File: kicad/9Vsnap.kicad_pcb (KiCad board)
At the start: 2 copper layers, 26 x 17 mm, 11 parts, among them P1 9V_IN, P2 OUT, U1 LM317EMP

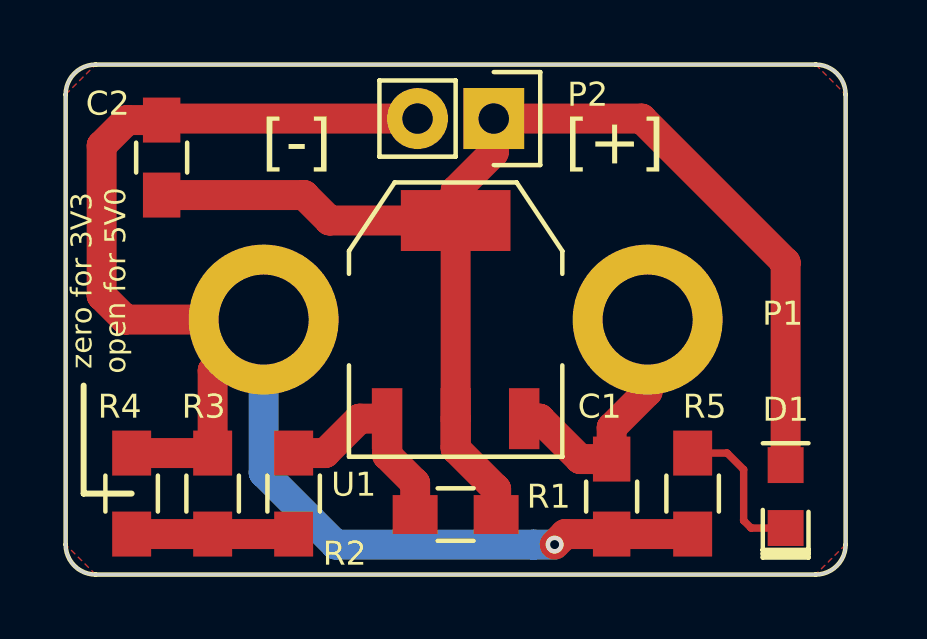
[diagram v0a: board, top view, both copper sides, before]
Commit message: Done. Gerbers ready
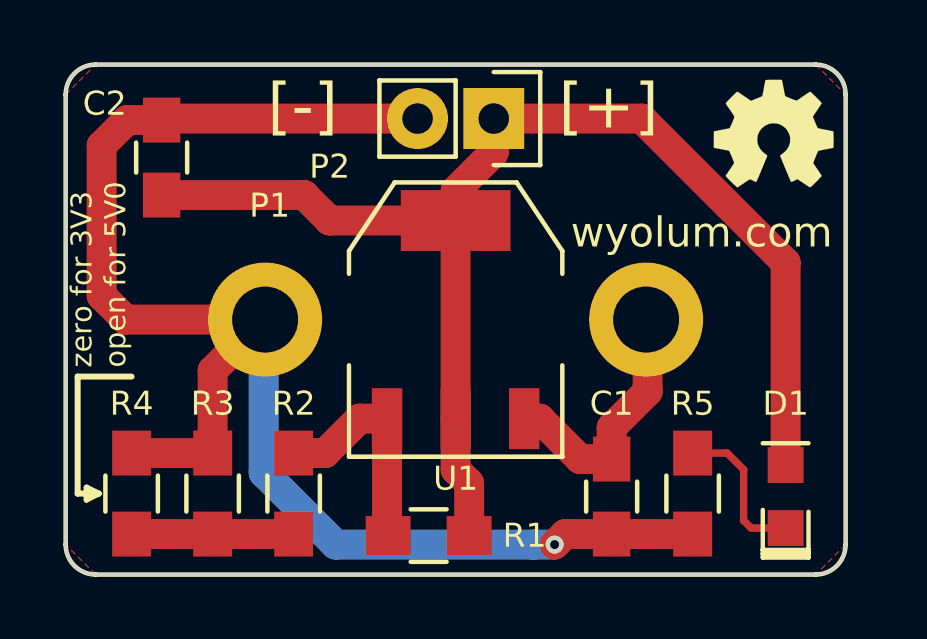
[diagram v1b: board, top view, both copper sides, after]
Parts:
- added G***: LOGO, 9Vsnap:OSHW_logo_notext, B.Cu at (100.0, 102.5)
- added G***: LOGO, 9Vsnap:OSHW_logo_notext, F.Cu at (110.6, 93.8)
- P1: footprint 9Vsnap:9V_clip -> 9Vsnap:9V_clip_968
- moved R1 1.14 mm to (99.1, 107.2)
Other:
- board text added: "github.com/wyolum"
- board text added: "hardware"
- board text added: "open source"
- board text added: "wyolum.com"
